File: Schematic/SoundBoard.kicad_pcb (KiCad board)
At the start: 2 copper layers, 56.5 x 74 mm, 60 parts, among them J1 Conn_ARM_JTAG_SWD_10, J2 Micro_SD_Card, J3 USB_B_Micro, SW1 SW_Push, SW2 SW_Push, U1 STM32F427VGTx, U2 AH1806-W, U3 FT232RL, U4 TPA301DR, U5 MCP73812T-420I-OT, U6 STC3100IST, U7 MIC5504-3.3YM5, U8 MIC5504-3.3YM5

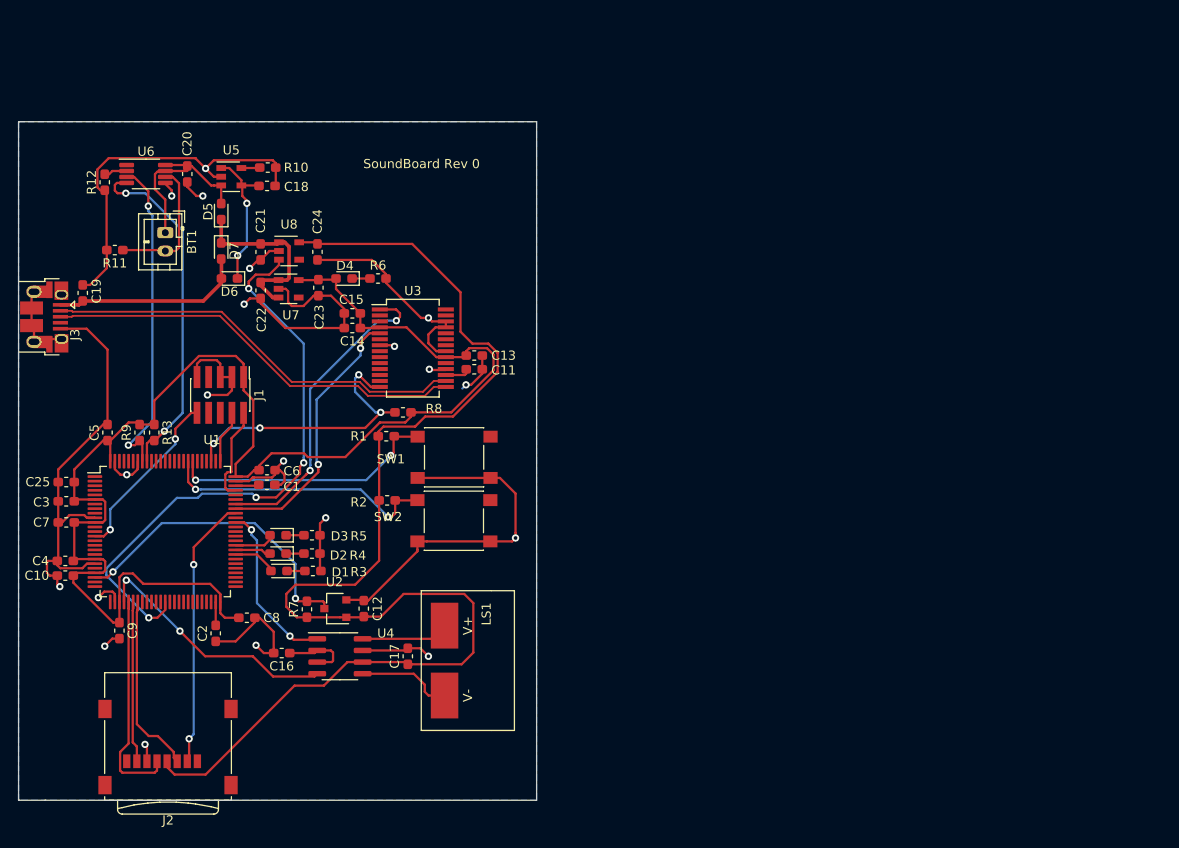
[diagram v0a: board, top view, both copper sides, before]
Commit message: Add gerbers
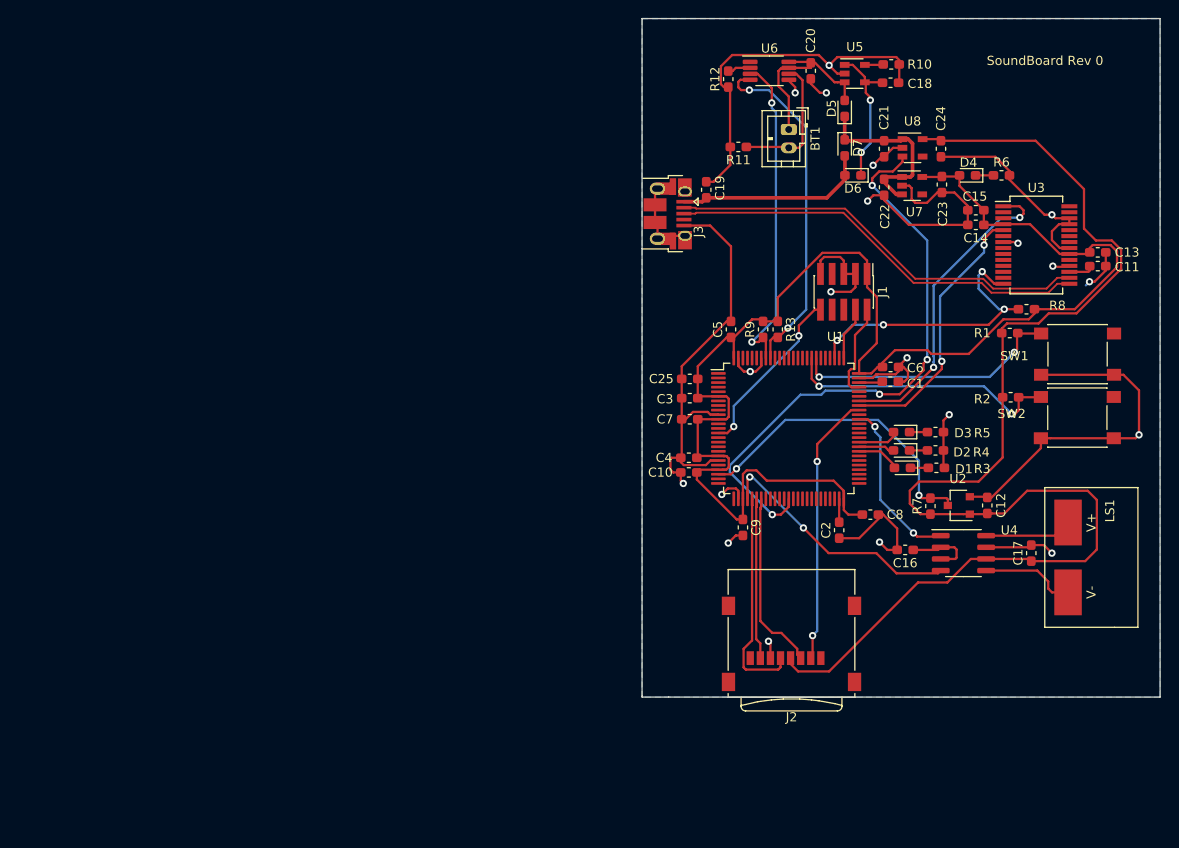
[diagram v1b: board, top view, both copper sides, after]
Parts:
- moved BT1 68.9 mm to (134.3, 67.8)
- moved C2 68.9 mm to (139.8, 111.5)
- moved C9 68.9 mm to (129.3, 111.2)
- moved D4 68.9 mm to (153.8, 72.8)
- moved D6 68.9 mm to (141.3, 72.8)
- moved J1 68.9 mm to (140.3, 85.5)
- moved LS1 68.9 mm to (167.3, 113.2)
- moved R11 68.9 mm to (128.8, 69.7)
- moved R4 68.9 mm to (150.3, 102.8)
- moved R5 68.9 mm to (150.3, 100.8)
- moved SW1 68.9 mm to (165.8, 92.2)
- moved SW2 68.9 mm to (165.8, 99.2)
- moved U1 68.9 mm to (134.3, 100.3)
- moved U3 68.9 mm to (161.3, 80.3)
- moved U8 68.9 mm to (147.8, 69.8)
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
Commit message: Perform layout
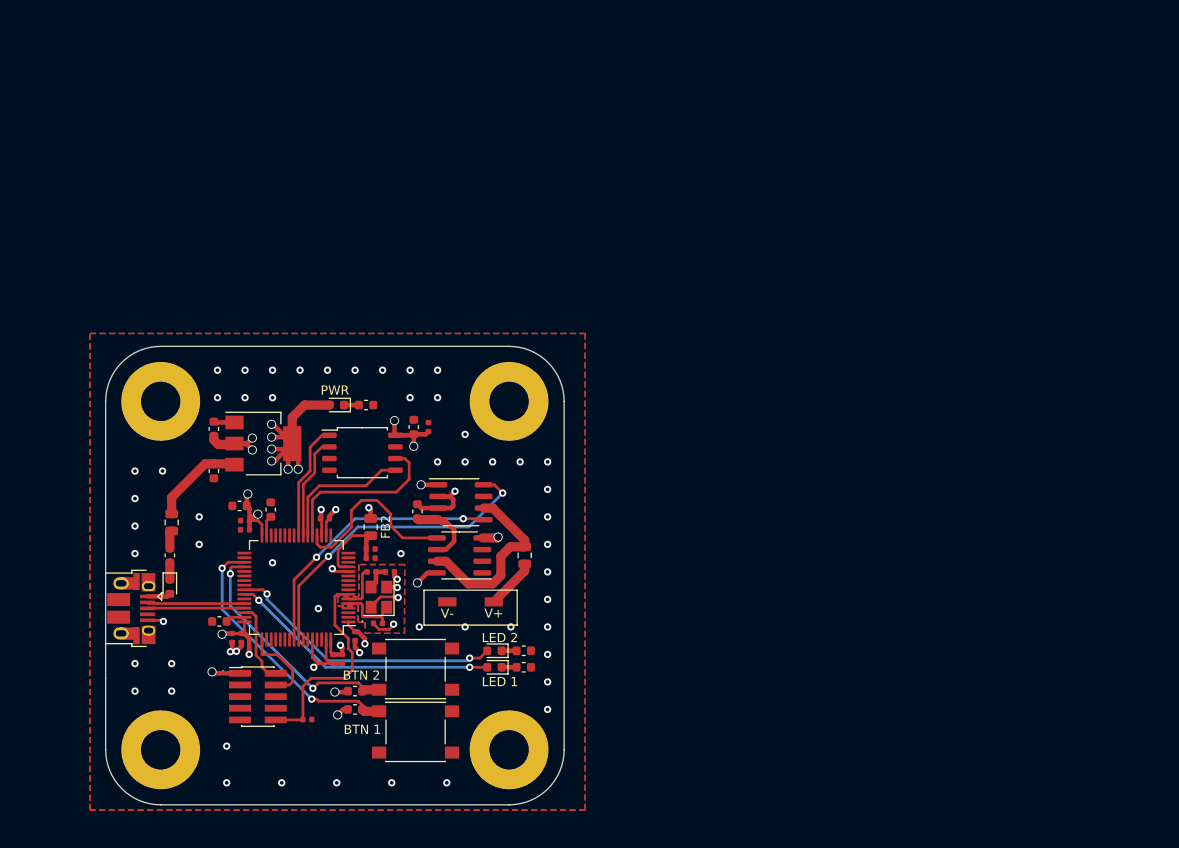
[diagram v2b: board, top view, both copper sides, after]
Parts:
- removed BT1: Battery_Cell, Connector_JST:JST_PH_B2B-PH-K_1x02_P2.00mm_Vertical
- removed C22, C23, C24: 1uF, Capacitor_SMD:C_0603_1608Metric_Pad1.05x0.95mm_HandSolder
- removed C25: 100nF, Capacitor_SMD:C_0603_1608Metric_Pad1.05x0.95mm_HandSolder
- removed D5, D6, D7: D_Schottky, Diode_SMD:D_0603_1608Metric_Pad1.05x0.95mm_HandSolder
- removed J3: USB_B_Micro, Connector_USB:USB_Micro-B_Amphenol_10103594-0001LF_Horizontal
- removed R10: 2K, Resistor_SMD:R_0603_1608Metric_Pad1.05x0.95mm_HandSolder
- removed R11: 10m, Resistor_SMD:R_0603_1608Metric_Pad1.05x0.95mm_HandSolder
- removed R12: 200k, Resistor_SMD:R_0603_1608Metric_Pad1.05x0.95mm_HandSolder
- removed R13, R9: 10K, Resistor_SMD:R_0603_1608Metric_Pad1.05x0.95mm_HandSolder
- removed R8: 10k, Resistor_SMD:R_0603_1608Metric_Pad1.05x0.95mm_HandSolder
- removed U6: STC3100IST, Package_SO:MSOP-8_3x3mm_P0.65mm
- removed U7, U8: MIC5504-3.3YM5, Package_TO_SOT_SMD:SOT-23-5
- added F1: 1A, Fuse:Fuse_0603_1608Metric, F.Cu at (66.8, 114.2)
- added FB1: Ferrite_Bead, Inductor_SMD:L_0805_2012Metric, F.Cu at (67.0, 110.6)
- added FB2: Ferrite_Bead_Small, Inductor_SMD:L_0805_2012Metric, F.Cu at (88.7, 111.1)
- added H1: MountingHole_Pad, MountingHole:MountingHole_4.3mm_M4_Pad, F.Cu at (103.8, 97.4)
- added H2: MountingHole_Pad, MountingHole:MountingHole_4.3mm_M4_Pad, F.Cu at (65.8, 135.4)
- added H3: MountingHole_Pad, MountingHole:MountingHole_4.3mm_M4_Pad, F.Cu at (65.8, 97.4)
- added H4: MountingHole_Pad, MountingHole:MountingHole_4.3mm_M4_Pad, F.Cu at (103.8, 135.4)
- added Y1: 25Mhz, Crystal:Crystal_SMD_3225-4Pin_3.2x2.5mm, F.Cu at (89.6, 118.8)
- C1: value 2.2uF -> 10u; footprint Capacitor_SMD:C_0603_1608Metric_Pad1.05x0.95mm_HandSolder -> Capacitor_SMD:C_0603_1608Metric
- C10: value 4.7uF -> 100n; footprint Capacitor_SMD:C_0603_1608Metric_Pad1.05x0.95mm_HandSolder -> Capacitor_SMD:C_0402_1005Metric
- C11, C12, C13, C14, C16, C19, C8, C9: value 100nF -> 100n; footprint Capacitor_SMD:C_0603_1608Metric_Pad1.05x0.95mm_HandSolder -> Capacitor_SMD:C_0402_1005Metric
- C15: value 4.7uF -> 10n; footprint Capacitor_SMD:C_0603_1608Metric_Pad1.05x0.95mm_HandSolder -> Capacitor_SMD:C_0402_1005Metric
- C17, C21: value 1uF -> 100n; footprint Capacitor_SMD:C_0603_1608Metric_Pad1.05x0.95mm_HandSolder -> Capacitor_SMD:C_0402_1005Metric
- C18: value 1uF -> 10p; footprint Capacitor_SMD:C_0603_1608Metric_Pad1.05x0.95mm_HandSolder -> Capacitor_SMD:C_0805_2012Metric
- C2: value 2.2uF -> 20p; footprint Capacitor_SMD:C_0603_1608Metric_Pad1.05x0.95mm_HandSolder -> Capacitor_SMD:C_0402_1005Metric
- C20, C4, C7: value 100nF -> 10u; footprint Capacitor_SMD:C_0603_1608Metric_Pad1.05x0.95mm_HandSolder -> Capacitor_SMD:C_0603_1608Metric
- C3: value 100nF -> 20p; footprint Capacitor_SMD:C_0603_1608Metric_Pad1.05x0.95mm_HandSolder -> Capacitor_SMD:C_0402_1005Metric
- C5, C6: value 100nF -> 2.2u; footprint Capacitor_SMD:C_0603_1608Metric_Pad1.05x0.95mm_HandSolder -> Capacitor_SMD:C_0603_1608Metric
- D1: value LED -> D_Schottky; footprint Diode_SMD:D_0603_1608Metric_Pad1.05x0.95mm_HandSolder -> Diode_SMD:D_0603_1608Metric
- D2, D3, D4: footprint Diode_SMD:D_0603_1608Metric_Pad1.05x0.95mm_HandSolder -> LED_SMD:LED_0603_1608Metric
- J1: value Conn_ARM_JTAG_SWD_10 -> USB_B_Micro; footprint Connector_PinHeader_1.27mm:PinHeader_2x05_P1.27mm_Vertical_SMD -> Connector_USB:USB_Micro-B_Amphenol_10103594-0001LF_Horizontal
- J2: value Micro_SD_Card -> Conn_ARM_JTAG_SWD_10; footprint Connector_Card:microSD_HC_Wuerth_693072010801 -> Connector_PinHeader_1.27mm:PinHeader_2x05_P1.27mm_Vertical_SMD
- R1: value 10K -> 220; footprint Resistor_SMD:R_0603_1608Metric_Pad1.05x0.95mm_HandSolder -> Resistor_SMD:R_0603_1608Metric
- R2: value 10K -> 10k; footprint Resistor_SMD:R_0603_1608Metric_Pad1.05x0.95mm_HandSolder -> Resistor_SMD:R_0603_1608Metric
- R3: value 150 -> 10k; footprint Resistor_SMD:R_0603_1608Metric_Pad1.05x0.95mm_HandSolder -> Resistor_SMD:R_0603_1608Metric
- R4, R6: value 150 -> 220; footprint Resistor_SMD:R_0603_1608Metric_Pad1.05x0.95mm_HandSolder -> Resistor_SMD:R_0603_1608Metric
- R5: footprint Resistor_SMD:R_0603_1608Metric_Pad1.05x0.95mm_HandSolder -> Resistor_SMD:R_0402_1005Metric
- R7: footprint Resistor_SMD:R_0603_1608Metric_Pad1.05x0.95mm_HandSolder -> Resistor_SMD:R_0603_1608Metric
- U1: value STM32F427VGTx -> AMS1117-3.3; footprint Package_QFP:LQFP-100_14x14mm_P0.5mm -> Package_TO_SOT_SMD:SOT-223-3_TabPin2
- U2: value AH1806-W -> STM32F405RGTx; footprint Package_TO_SOT_SMD:SC-59 -> Package_QFP:LQFP-64_10x10mm_P0.5mm
- U3: value FT232RL -> MCP4021-xxxxSN; footprint Package_SO:SSOP-28_5.3x10.2mm_P0.65mm -> Package_SO:SOIC-8_3.9x4.9mm_P1.27mm
- U4: value TPA301DR -> LM4562
- U5: value MCP73812T-420I-OT -> W25Q128JVS; footprint Package_TO_SOT_SMD:SOT-23-5 -> Package_SO:SOIC-8_5.23x5.23mm_P1.27mm
- moved C11 101.8 mm to (74.6, 123.2), turned to 270 degrees
- moved C21 88.5 mm to (81.8, 132.1), turned to 0 degrees
- moved C17 87.6 mm to (73.6, 123.2), turned to 270 degrees
- moved C13 85.6 mm to (88.7, 113.5)
- moved J1 85.0 mm to (62.6, 120.0)
- moved C14 84.6 mm to (84.6, 125.5), turned to 270 degrees
- moved SW1 83.1 mm to (93.6, 133.4), turned to 0 degrees
- moved D1 80.9 mm to (66.8, 117.6), turned to 270 degrees
- moved R2 79.2 mm to (87.0, 131.0)
- moved C6 78.3 mm to (72.2, 121.4), turned to 180 degrees
- moved SW2 77.2 mm to (93.6, 126.6)
- moved C15 76.1 mm to (88.7, 114.5), turned to 0 degrees
- moved C1 74.4 mm to (71.6, 105.0), turned to 270 degrees
- moved R6 73.5 mm to (105.4, 124.6)
- moved D4 73.2 mm to (102.2, 124.6)
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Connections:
- C1 pad 1: GND -> Net-(C1-Pad1)
- C1 pad 2: Net-(C1-Pad2) -> GND
- C10 pad 1: /MCU/VDD -> +3V3
- C11 pad 1: Net-(C11-Pad1) -> +3V3
- C12 pad 1: /Audio/V1 -> +3V3
- C13 pad 1: /MCU/VDD -> +3.3VA
- C14 pad 1: /MCU/VDD -> +3V3
- C15 pad 1: /MCU/VDD -> +3.3VA
- C16 pad 1: Net-(C16-Pad1) -> +3V3
- C17 pad 1: /Audio/V1 -> +3V3
- C18 pad 2: GND -> Net-(C18-Pad2)
- C19 pad 1: Net-(C19-Pad1) -> +3V3
- C2 pad 1: GND -> /OSC_IN
- C2 pad 2: Net-(C2-Pad2) -> GND
- C20 pad 1: Net-(BT1-Pad1) -> +3V3
- C21 pad 1: /Power/VRAW -> /NRESET
- C3 pad 1: /MCU/VDD -> Net-(C3-Pad1)
- C4 pad 1: /MCU/VDD -> +3V3
- C5 pad 1: /MCU/VDD -> Net-(C5-Pad1)
- C6 pad 1: /MCU/VDD -> Net-(C6-Pad1)
- C7 pad 1: GND -> +3V3
- C7 pad 2: /MCU/VDD -> GND
- C8 pad 1: /MCU/VDD -> +3V3
- C9 pad 1: /MCU/VDD -> +3V3
- D1 pad 2: Net-(D1-Pad2) -> VDD
- D2 pad 2: Net-(D2-Pad2) -> +3V3
- D3 pad 2: Net-(D3-Pad2) -> /LED_1
- D4 pad 2: /MCU/VDD -> /LED_2
- J1 pad 1: /MCU/VDD -> VDD
- J1 pad 2: Net-(J1-Pad2) -> /USBD_N
- J1 pad 3: GND -> /USBD_P
- J2 pad 1: Net-(J2-Pad1) -> +3V3
- J2 pad 2: /MCU/SD_SELECT -> /SWDIO
- J2 pad 3: /MCU/SD_MOSI -> GND
- J2 pad 4: /Audio/V1 -> /SWCLK
- J2 pad 5: /MCU/SD_CLK -> GND
- J2 pad 6: GND -> Net-(J2-Pad6)
- J2 pad 7: /MCU/SD_MISO -> Net-(J2-Pad7)
- J2 pad 9: Net-(J2-Pad9) -> GND
- LS1 pad 1: Net-(LS1-Pad1) -> Net-(C18-Pad1)
- LS1 pad 2: Net-(LS1-Pad2) -> GND
- R1 pad 1: /Audio/V1 -> Net-(D2-Pad1)
- R1 pad 2: Net-(R1-Pad2) -> GND
- R2 pad 1: /Audio/V1 -> +3V3
- R2 pad 2: Net-(R2-Pad2) -> /BTN_1
- R3 pad 1: Net-(D1-Pad1) -> +3V3
- R3 pad 2: GND -> /BTN_2
- R4 pad 1: Net-(D2-Pad1) -> Net-(D3-Pad1)
- R5 pad 1: Net-(D3-Pad1) -> /OSC_OUT
- R5 pad 2: GND -> Net-(C3-Pad1)
- R7 pad 1: /Audio/V1 -> Net-(R7-Pad1)
- R7 pad 2: /MCU/HALL_SENSOR -> GND
- SW1 pad 1: GND -> /BTN_1
- SW1 pad 2: Net-(R1-Pad2) -> GND
- SW2 pad 1: GND -> /BTN_2
- SW2 pad 2: Net-(R2-Pad2) -> GND
- U1 pad 1: Net-(U1-Pad1) -> GND
- U1 pad 2: Net-(U1-Pad2) -> +3V3
- U1 pad 3: Net-(U1-Pad3) -> Net-(C1-Pad1)
- U2 pad 1: /Audio/V1 -> +3V3
- U2 pad 2: GND -> Net-(U2-Pad2)
- U2 pad 3: /MCU/HALL_SENSOR -> Net-(U2-Pad3)
- U3 pad 1: /MCU/RX_TO_STM32 -> +3V3
- U3 pad 2: Net-(U3-Pad2) -> GND
- U3 pad 3: Net-(U3-Pad3) -> GND
- U3 pad 4: /MCU/VDD -> Net-(R7-Pad1)
- U3 pad 5: /MCU/TX_FROM_STM32 -> /POT_CS_N
- U3 pad 6: Net-(U3-Pad6) -> Net-(C18-Pad2)
- U3 pad 7: GND -> Net-(U3-Pad7)
- U3 pad 8: (no net) -> /POT_UD
- U4 pad 1: /Audio/SHUTDOWN -> (no net)
- U4 pad 2: Net-(C16-Pad1) -> (no net)
- U4 pad 3: Net-(C16-Pad1) -> (no net)
- U4 pad 4: /Audio/AUDIO_FROM_DAC -> GND
- U4 pad 5: Net-(LS1-Pad2) -> /DAC_OUT
- U4 pad 6: /Audio/V1 -> Net-(R7-Pad1)
- U4 pad 7: GND -> Net-(C18-Pad2)
- U4 pad 8: Net-(LS1-Pad1) -> +3V3
- U5 pad 1: Net-(C18-Pad1) -> /SPI_FLASH_CS
- U5 pad 2: GND -> /SPI_MOSI
- U5 pad 3: Net-(BT1-Pad1) -> Net-(U5-Pad3)
- U5 pad 4: Net-(C18-Pad1) -> GND
- U5 pad 5: Net-(R10-Pad2) -> /SPI_MISO
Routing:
- net GND: track 249.1 -> 41.0 mm, vias 20 -> 65
- net /MCU/VDD: track 158.2 -> 0.00 mm
- net /Audio/V1: track 142.9 -> 0.00 mm
- net +3V3: track 0.00 -> 74.9 mm, vias 0 -> 23
- net /MCU/V1_EN: track 64.3 -> 0.00 mm, vias 4 -> 0
- net /MCU/USB_N: track 46.2 -> 0.00 mm
- net /MCU/USB_P: track 46.1 -> 0.00 mm
- net /MCU/FUEL_SCL: track 38.3 -> 0.00 mm, vias 2 -> 0
- net /MCU/FUEL_SDA: track 35.8 -> 0.00 mm, vias 2 -> 0
- net /POT_UD: track 0.00 -> 34.7 mm, vias 0 -> 2
- net /MCU/RX_TO_STM32: track 34.4 -> 0.00 mm, vias 2 -> 0
- net /MCU/HALL_SENSOR: track 33.9 -> 0.00 mm, vias 2 -> 0
- net /MCU/FTDI_PWR_EN: track 31.8 -> 0.00 mm, vias 4 -> 0
- net /LED_2: track 0.00 -> 30.5 mm, vias 0 -> 2
- net Net-(R2-Pad2): track 30.4 -> 0.00 mm, vias 2 -> 0
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- added copper zone on PWR, net +3V3
- added copper zone on F.Cu, net GND
- added copper zone on GND, net GND
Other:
- board size 56.5 x 74 mm -> 50 x 50 mm
- copper layers 2 -> 4
- board text added: "."
- board text added: "BTN 1"
- board text added: "BTN 2"
- board text added: "DESIGNED BY JOE PERRI"
- board text added: "JLCJLCJLC"
- board text added: "LED 1"
- board text added: "LED 2"
- board text added: "PWR"
- board text added: "SOUNDBOARD REV 1.0"
- board text removed: "SoundBoard Rev 0"

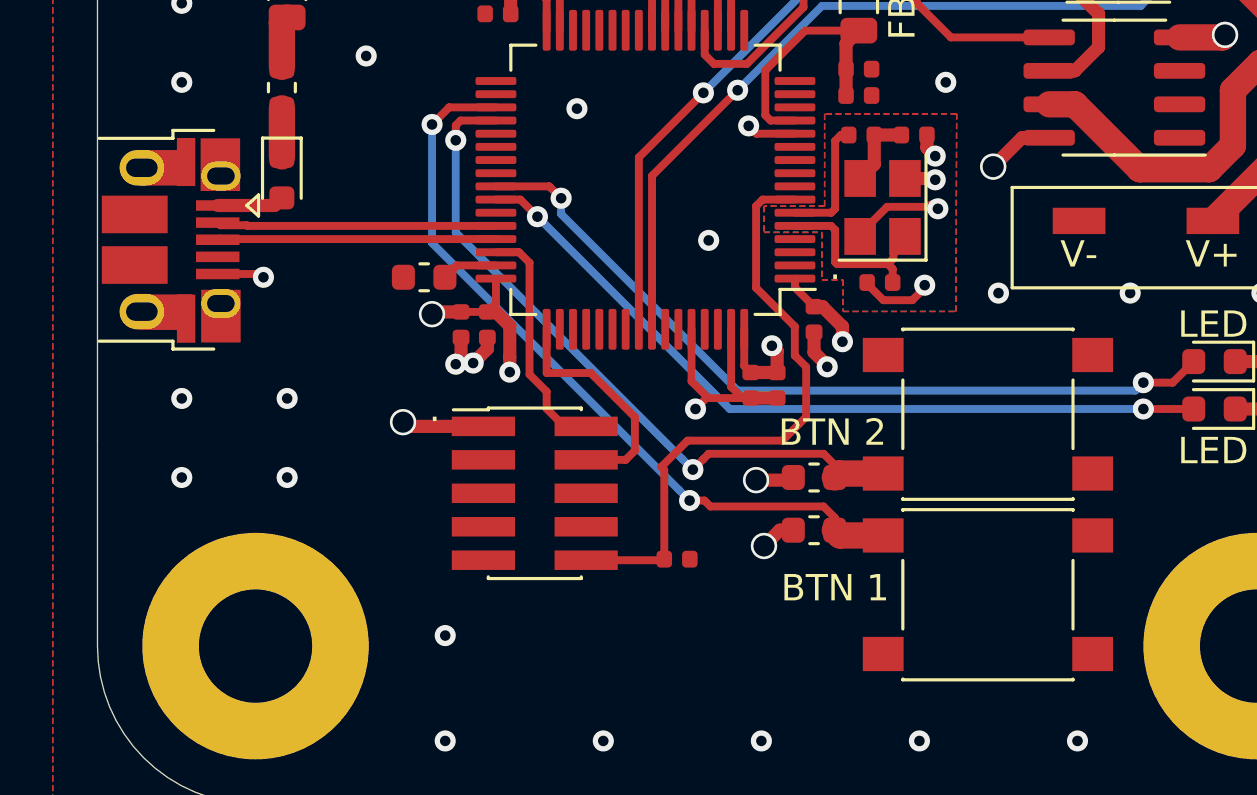
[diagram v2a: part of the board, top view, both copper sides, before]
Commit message: Update gerbers
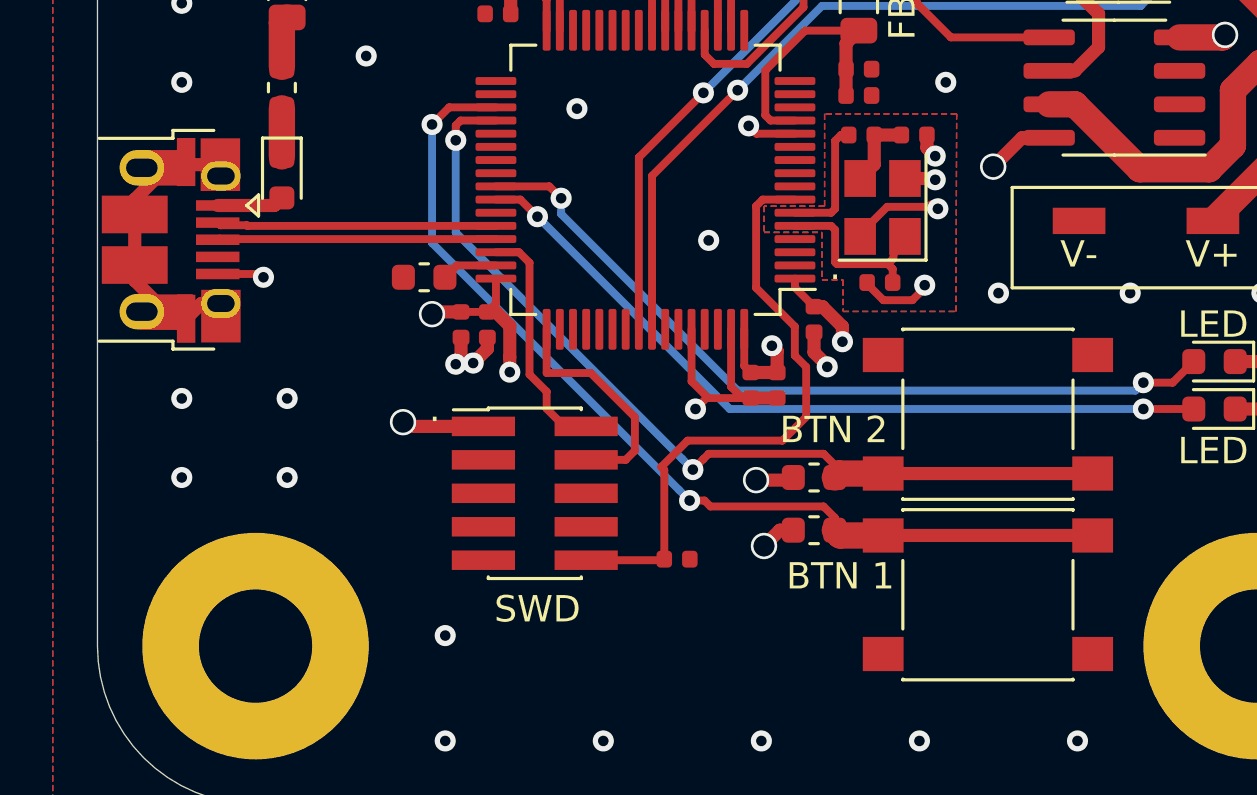
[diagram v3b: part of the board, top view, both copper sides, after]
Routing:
- net Net-(J1-Pad6): track 0.00 -> 10.1 mm
- net /BTN_2: track 26.6 -> 34.5 mm
- net /BTN_1: track 29.2 -> 37.1 mm
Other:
- board text added: "SWD"
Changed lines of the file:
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@@
   (general
     (thickness 1.6)
-    (drawings 19)
-    (tracks 435)
+    (drawings 20)
+    (tracks 447)
     (zones 0)
     (modules 50)
@@
     (47 F.CrtYd user)
     (48 B.Fab user)
-    (49 F.Fab user hide)
+    (49 F.Fab user)
   )
   (setup
@@
     (tags capacitor)
     (attr smd)
-    (fp_text reference C21 (at 0.4 1.3) (layer F.Fab)
+    (fp_text reference C21 (at -0.05 -0.85) (layer F.Fab)
       (effects (font (size 1 1) (thickness 0.15)))
     )
@@
     )
   )
+  (gr_text "SWD\n" (at 76.5 134) (layer F.SilkS)
+    (effects (font (size 1 1) (thickness 0.15)))
+  )
   (gr_text "DESIGNED BY JOE PERRI\n" (at 85 137.2) (layer B.SilkS)
     (effects (font (size 1 1) (thickness 0.15)) (justify mirror))
@@
     (effects (font (size 1 1) (thickness 0.15)))
   )
-  (gr_text "BTN 2\n\n" (at 87.7 128.1) (layer F.SilkS)
+  (gr_text "BTN 2\n\n" (at 87.75 128) (layer F.SilkS)
     (effects (font (size 1 1) (thickness 0.15)))
   )
-  (gr_text "BTN 1\n" (at 87.8 133.2) (layer F.SilkS)
+  (gr_text "BTN 1\n" (at 88 132.75) (layer F.SilkS)
     (effects (font (size 1 1) (thickness 0.15)))
   )
@@
   (segment (start 72.5 120.098397) (end 81.876266 129.474663) (width 0.3) (layer B.Cu) (net 26))
   (via (at 82.276265 129.874662) (size 0.8) (drill 0.4) (layers F.Cu B.Cu) (net 26))
+  (segment (start 89.625 131.2) (end 97.575 131.2) (width 0.5) (layer F.Cu) (net 26))
   (segment (start 87.9375 128.85) (end 87.7875 129) (width 1) (layer F.Cu) (net 27))
   (segment (start 89.625 128.85) (end 87.9375 128.85) (width 1) (layer F.Cu) (net 27))
@@
   (segment (start 73.4 116.2) (end 73.4 119.7) (width 0.3) (layer B.Cu) (net 27))
   (segment (start 82.000001 128.300001) (end 82.4 128.7) (width 0.3) (layer B.Cu) (net 27))
+  (segment (start 90.9 128.85) (end 97.575 128.85) (width 0.5) (layer F.Cu) (net 27))
+  (segment (start 89.625 128.85) (end 90.9 128.85) (width 0.5) (layer F.Cu) (net 27))
   (segment (start 88.02 116) (end 88.315 116) (width 0.3) (layer F.Cu) (net 28))
   (segment (start 87.799999 116.220001) (end 88.02 116) (width 0.3) (layer F.Cu) (net 28))
@@
   (segment (start 65.470001 119.424999) (end 64.464999 119.424999) (width 0.3) (layer F.Cu) (net 75))
   (segment (start 65.495002 119.45) (end 65.470001 119.424999) (width 0.3) (layer F.Cu) (net 75))
+  (segment (start 61.215 120.935) (end 61.215 119.015) (width 0.5) (layer F.Cu) (net 76))
+  (segment (start 61.215 118.445) (end 62.415 117.245) (width 0.5) (layer F.Cu) (net 76))
+  (segment (start 61.215 119.015) (end 61.215 118.445) (width 0.5) (layer F.Cu) (net 76))
+  (segment (start 61.215 121.525) (end 62.415 122.725) (width 0.5) (layer F.Cu) (net 76))
+  (segment (start 61.215 120.935) (end 61.215 121.525) (width 0.5) (layer F.Cu) (net 76))
+  (segment (start 63.745 122.395) (end 63.165 122.975) (width 0.5) (layer F.Cu) (net 76))
+  (segment (start 64.485 122.395) (end 63.745 122.395) (width 0.5) (layer F.Cu) (net 76))
+  (segment (start 62.535 117.125) (end 62.415 117.245) (width 0.5) (layer F.Cu) (net 76))
+  (segment (start 64.465 117.125) (end 62.535 117.125) (width 0.5) (layer F.Cu) (net 76))
   (zone (net 1) (net_name GND) (layer GND) (hatch edge 0.508)
     (connect_pads (clearance 0.508))
